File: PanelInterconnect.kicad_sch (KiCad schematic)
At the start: 10 parts, among them J1 Conn_01x10, J3 Conn_01x30

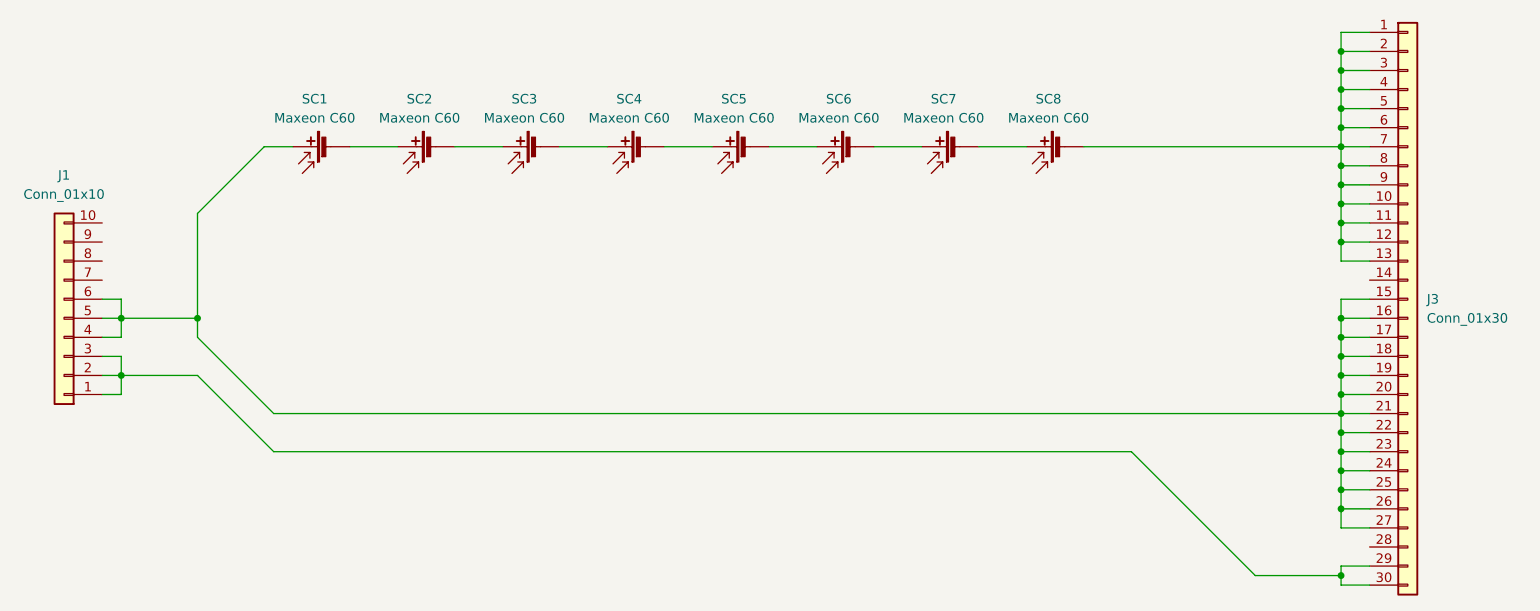
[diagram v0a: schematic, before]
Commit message: Cleaning up layout
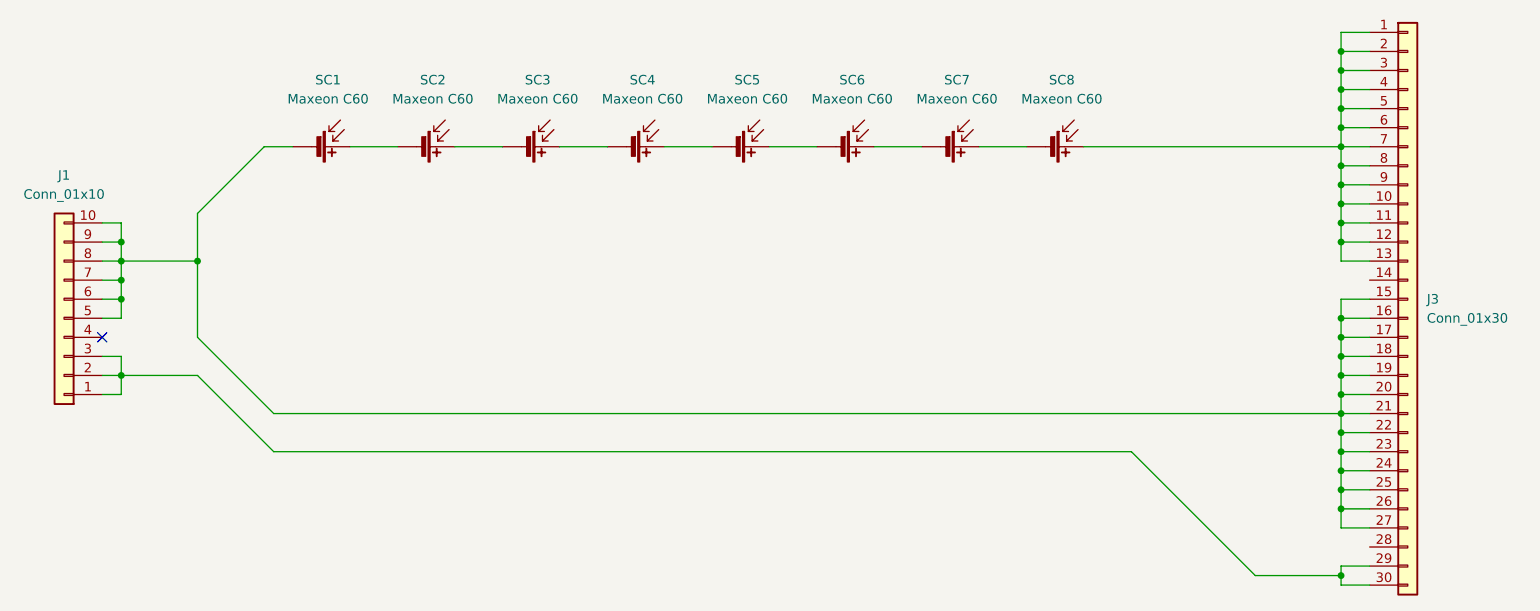
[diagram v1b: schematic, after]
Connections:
- net at SC4.1 (+): now also SC5.2 (-); no longer SC3.2 (-)
- net at SC4.2 (-): now also SC3.1 (+); no longer SC5.1 (+)
- net at SC7.1 (+): now also SC8.2 (-); no longer SC6.2 (-)
- net at SC7.2 (-): now also SC6.1 (+); no longer SC8.1 (+)
- net at J1.5 (Pin_5), J1.6 (Pin_6), J3.15 (Pin_15)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: now also J1.10 (Pin_10), J1.7 (Pin_7), J1.8 (Pin_8), J1.9 (Pin_9), SC1.2 (-); no longer J1.4 (Pin_4), SC1.1 (+)
- net at SC2.1 (+): now also SC3.2 (-); no longer SC1.2 (-)
- net at SC2.2 (-): now also SC1.1 (+); no longer SC3.1 (+)
- net at J3.1 (Pin_1), J3.10 (Pin_10), J3.11 (Pin_11)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: now also SC8.1 (+); no longer SC8.2 (-)
- new net: SC5.1 (+), SC6.2 (-)
- no-connect marks 0 -> 1
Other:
- moved on the sheet: SC1, SC2, SC3, SC4, SC5, SC6, SC7, SC8

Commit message: Finishing up backup interconnects
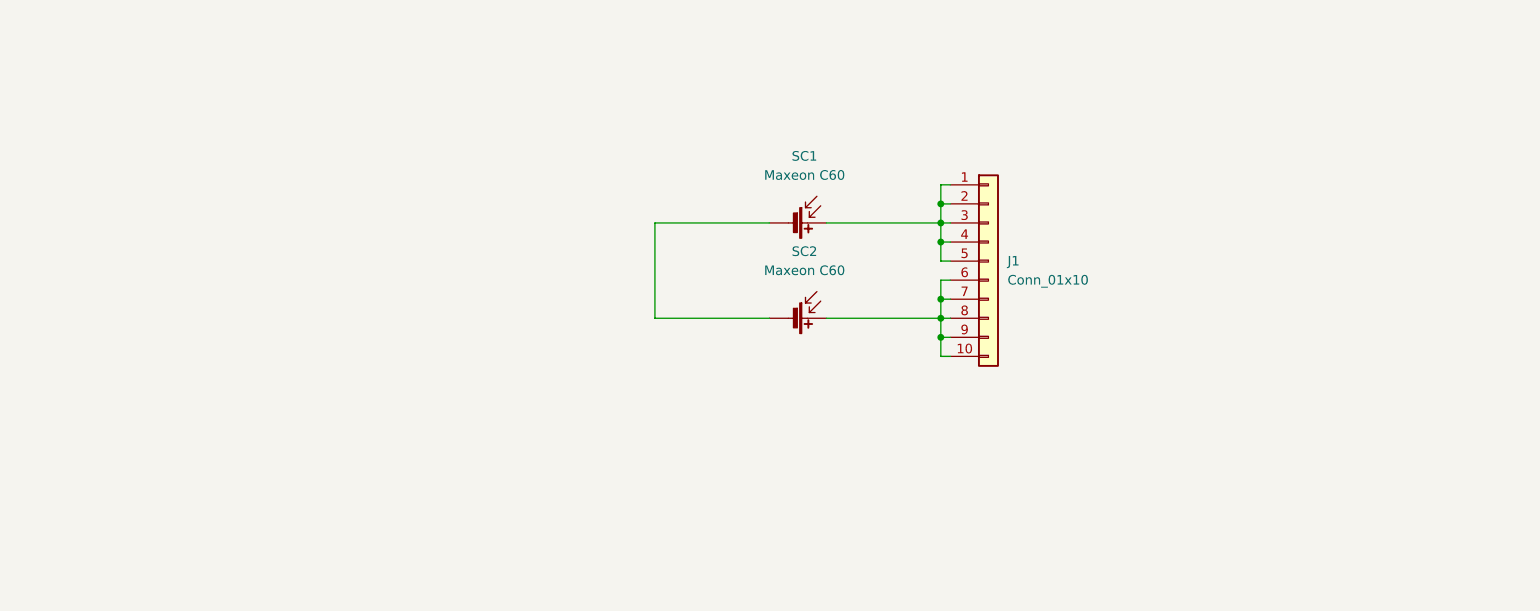
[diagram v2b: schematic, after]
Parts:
- removed J3: Conn_01x30, _PanelInterconnct:kyocera_fpc_01x30, symbol Connector_Generic:Conn_01x30
- removed SC3, SC4, SC5, SC6, SC7, SC8: Maxeon C60, _PanelInterconnct:maxeon_c60, symbol Device:Solar_Cell
- J1: footprint _PanelInterconnct:kyocera_fpc_01x10 -> _PanelInterconnects:tb4_10p
- SC1, SC2: footprint _PanelInterconnct:maxeon_c60 -> _PanelInterconnects:maxeon_c60
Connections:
- net at SC1.1 (+): now also J1.1 (Pin_1), J1.2 (Pin_2), J1.3 (Pin_3), J1.4 (Pin_4), J1.5 (Pin_5); no longer SC2.2 (-)
- net at J1.10 (Pin_10), J1.6 (Pin_6), J1.7 (Pin_7)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: now also SC2.1 (+); no longer J1.5 (Pin_5), SC1.2 (-)
- new net: SC1.2 (-), SC2.2 (-)
- no-connect marks 1 -> 0
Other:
- moved on the sheet: SC1
